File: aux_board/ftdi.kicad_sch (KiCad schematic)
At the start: 14 parts, among them U4 FT230XS

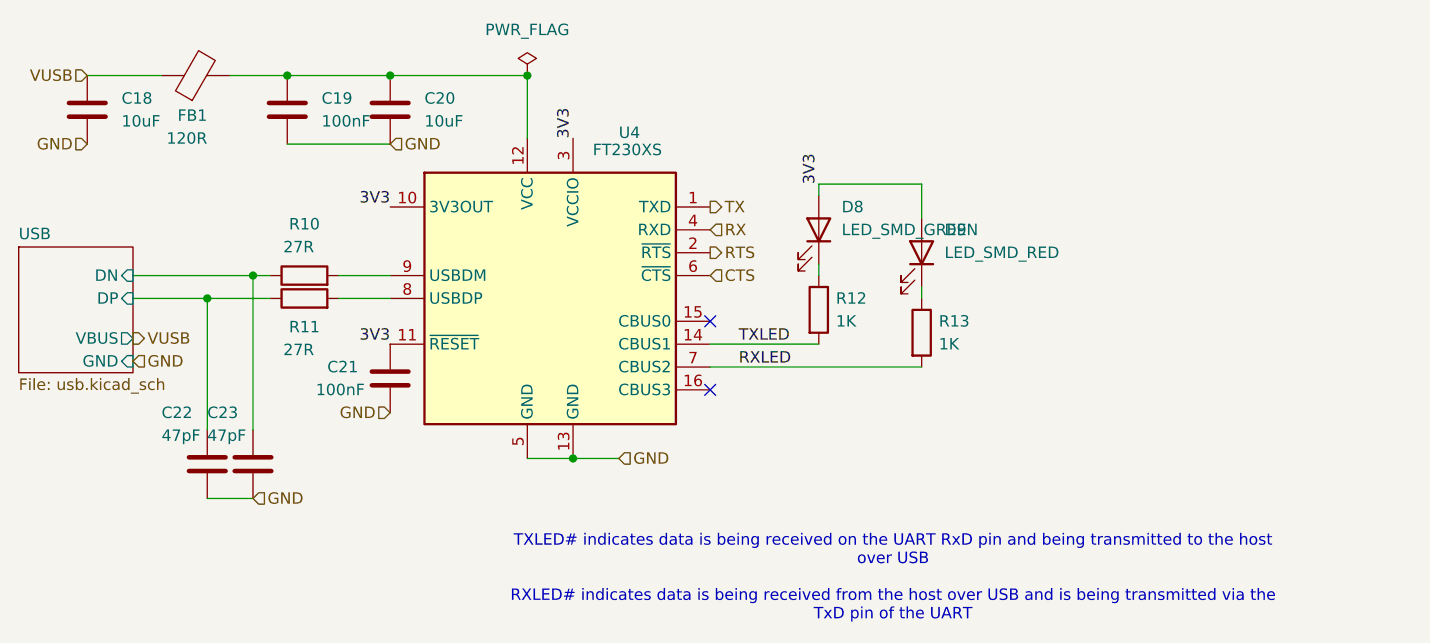
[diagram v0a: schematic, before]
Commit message: propate the changes to RF
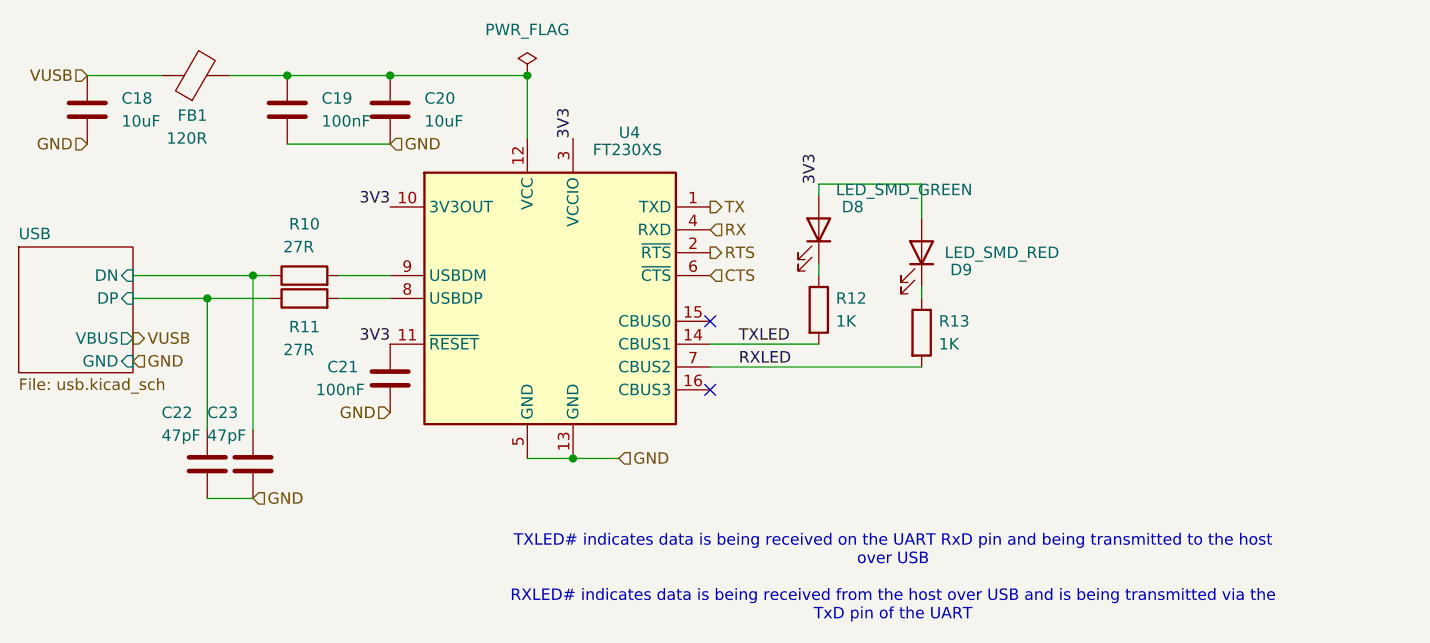
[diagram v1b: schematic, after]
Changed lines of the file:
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@@
 		)
 		(property "Value" "LED_SMD_GREEN"
-			(at 173.355 81.915 90)
+			(at 172.72 77.47 90)
 			(effects
 				(font
@@
 		)
 		(property "Voltage" "2"
-			(at 170.815 81.915 0)
-			(effects
-				(font
-					(size 1.27 1.27)
-				)
-				(hide yes)
-			)
-		)
-		(property "PARTREV" ""
-			(at 170.815 81.915 0)
-			(effects
-				(font
-					(size 1.27 1.27)
-				)
-				(hide yes)
-			)
-		)
-		(property "STANDARD" ""
 			(at 170.815 81.915 0)
 			(effects
@@
 			)
 		)
-		(property "PARTREV" ""
-			(at 123.19 68.58 0)
-			(effects
-				(font
-					(size 1.27 1.27)
-				)
-				(hide yes)
-			)
-		)
-		(property "STANDARD" ""
-			(at 123.19 68.58 0)
-			(effects
-				(font
-					(size 1.27 1.27)
-				)
-				(hide yes)
-			)
-		)
 		(pin "1"
 		)
@@
 		(dnp no)
 		(property "Reference" "D9"
-			(at 184.785 81.915 90)
+			(at 185.42 86.36 90)
 			(effects
 				(font
@@
 		)
 		(property "Voltage" "2"
-			(at 182.245 84.455 0)
-			(effects
-				(font
-					(size 1.27 1.27)
-				)
-				(hide yes)
-			)
-		)
-		(property "PARTREV" ""
-			(at 182.245 84.455 0)
-			(effects
-				(font
-					(size 1.27 1.27)
-				)
-				(hide yes)
-			)
-		)
-		(property "STANDARD" ""
 			(at 182.245 84.455 0)
 			(effects
@@
 			)
 		)
-		(property "PARTREV" ""
-			(at 170.815 90.805 0)
-			(effects
-				(font
-					(size 1.27 1.27)
-				)
-				(hide yes)
-			)
-		)
-		(property "STANDARD" ""
-			(at 170.815 90.805 0)
-			(effects
-				(font
-					(size 1.27 1.27)
-				)
-				(hide yes)
-			)
-		)
 		(pin "2"
 		)
@@
 			)
 		)
-		(property "PARTREV" ""
-			(at 140.97 89.535 0)
-			(effects
-				(font
-					(size 1.27 1.27)
-				)
-				(hide yes)
-			)
-		)
-		(property "STANDARD" ""
-			(at 140.97 89.535 0)
-			(effects
-				(font
-					(size 1.27 1.27)
-				)
-				(hide yes)
-			)
-		)
 		(pin "4"
 		)
@@
 		)
 		(property "Voltage" "50"
-			(at 107.95 107.95 0)
-			(effects
-				(font
-					(size 1.27 1.27)
-				)
-				(hide yes)
-			)
-		)
-		(property "PARTREV" ""
-			(at 107.95 107.95 0)
-			(effects
-				(font
-					(size 1.27 1.27)
-				)
-				(hide yes)
-			)
-		)
-		(property "STANDARD" ""
 			(at 107.95 107.95 0)
 			(effects
@@
 			)
 		)
-		(property "PARTREV" ""
-			(at 182.245 93.345 0)
-			(effects
-				(font
-					(size 1.27 1.27)
-				)
-				(hide yes)
-			)
-		)
-		(property "STANDARD" ""
-			(at 182.245 93.345 0)
-			(effects
-				(font
-					(size 1.27 1.27)
-				)
-				(hide yes)
-			)
-		)
 		(pin "2"
 		)
@@
 			)
 		)
-		(property "PARTREV" ""
-			(at 113.665 86.995 0)
-			(effects
-				(font
-					(size 1.27 1.27)
-				)
-				(hide yes)
-			)
-		)
-		(property "STANDARD" ""
-			(at 113.665 86.995 0)
-			(effects
-				(font
-					(size 1.27 1.27)
-				)
-				(hide yes)
-			)
-		)
 		(pin "1"
 		)
@@
 			)
 		)
-		(property "PARTREV" ""
-			(at 123.19 98.425 0)
-			(effects
-				(font
-					(size 1.27 1.27)
-				)
-				(hide yes)
-			)
-		)
-		(property "STANDARD" ""
-			(at 123.19 98.425 0)
-			(effects
-				(font
-					(size 1.27 1.27)
-				)
-				(hide yes)
-			)
-		)
 		(pin "1"
 		)
@@
 		)
 		(property "Voltage" "50"
-			(at 102.87 107.95 0)
-			(effects
-				(font
-					(size 1.27 1.27)
-				)
-				(hide yes)
-			)
-		)
-		(property "PARTREV" ""
-			(at 102.87 107.95 0)
-			(effects
-				(font
-					(size 1.27 1.27)
-				)
-				(hide yes)
-			)
-		)
-		(property "STANDARD" ""
 			(at 102.87 107.95 0)
 			(effects
@@
 			)
 		)
-		(property "PARTREV" ""
-			(at 111.76 68.58 0)
-			(effects
-				(font
-					(size 1.27 1.27)
-				)
-				(hide yes)
-			)
-		)
-		(property "STANDARD" ""
-			(at 111.76 68.58 0)
-			(effects
-				(font
-					(size 1.27 1.27)
-				)
-				(hide yes)
-			)
-		)
 		(pin "1"
 		)
@@
 			)
 		)
-		(property "PARTREV" ""
-			(at 89.535 68.58 0)
-			(effects
-				(font
-					(size 1.27 1.27)
-				)
-				(hide yes)
-			)
-		)
-		(property "STANDARD" ""
-			(at 89.535 68.58 0)
-			(effects
-				(font
-					(size 1.27 1.27)
-				)
-				(hide yes)
-			)
-		)
 		(pin "1"
 		)
@@
 			(at 113.665 89.535 0)
 			(effects
-				(font
-					(size 1.27 1.27)
-				)
-				(hide yes)
-			)
-		)
-		(property "PARTREV" ""
-			(at 113.665 89.535 0)
-			(effects
-				(font
-					(size 1.27 1.27)
-				)
-				(hide yes)
-			)
-		)
-		(property "STANDARD" ""
-			(at 113.665 89.535 0)
-			(effects
